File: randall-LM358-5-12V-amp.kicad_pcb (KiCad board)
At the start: 2 copper layers, 137.2 x 91.4 mm, 27 parts, among them J1 Barrel_Jack, M1 Fan_3pin, M2 Fan_3pin, Q1 TIP120, Q2 TIP120, U1 LM2674M-3.3, U2 LM358, U3 Z-Uno

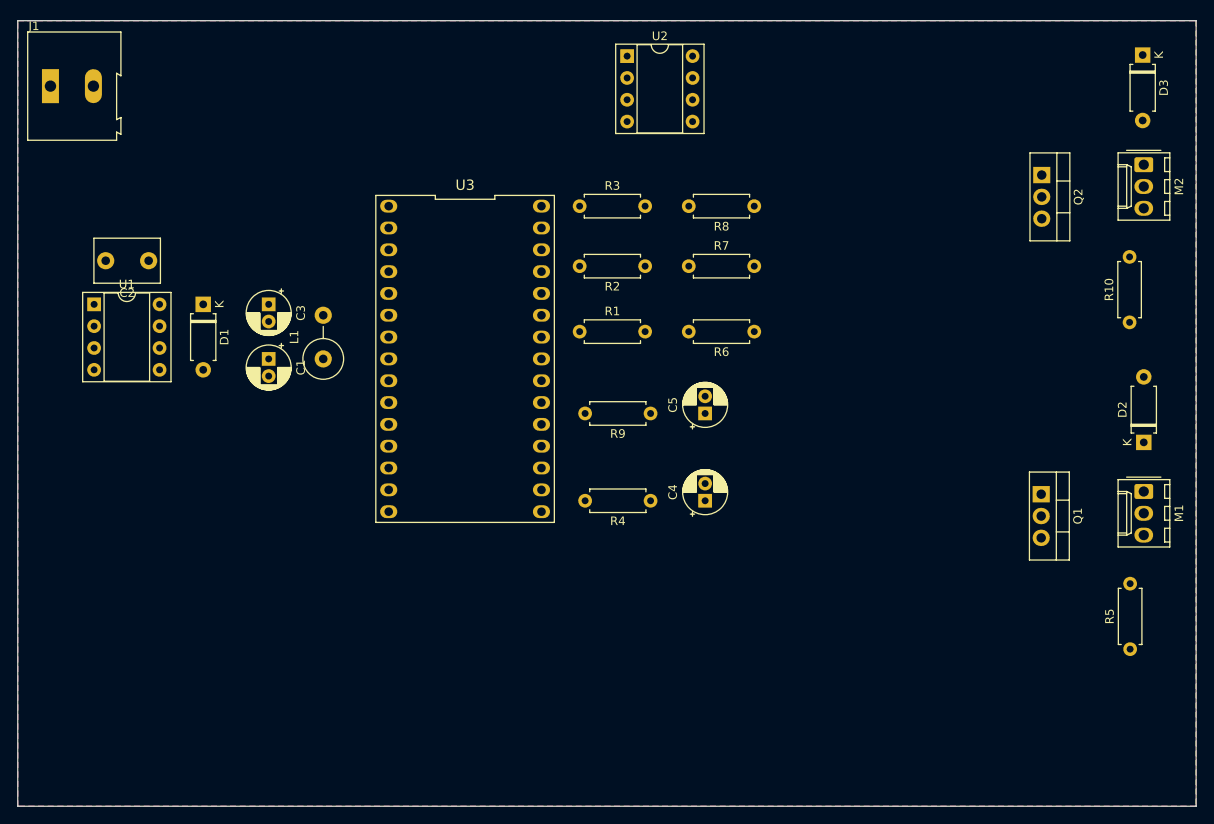
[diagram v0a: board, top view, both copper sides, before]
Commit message: This is it, make no mistake about it
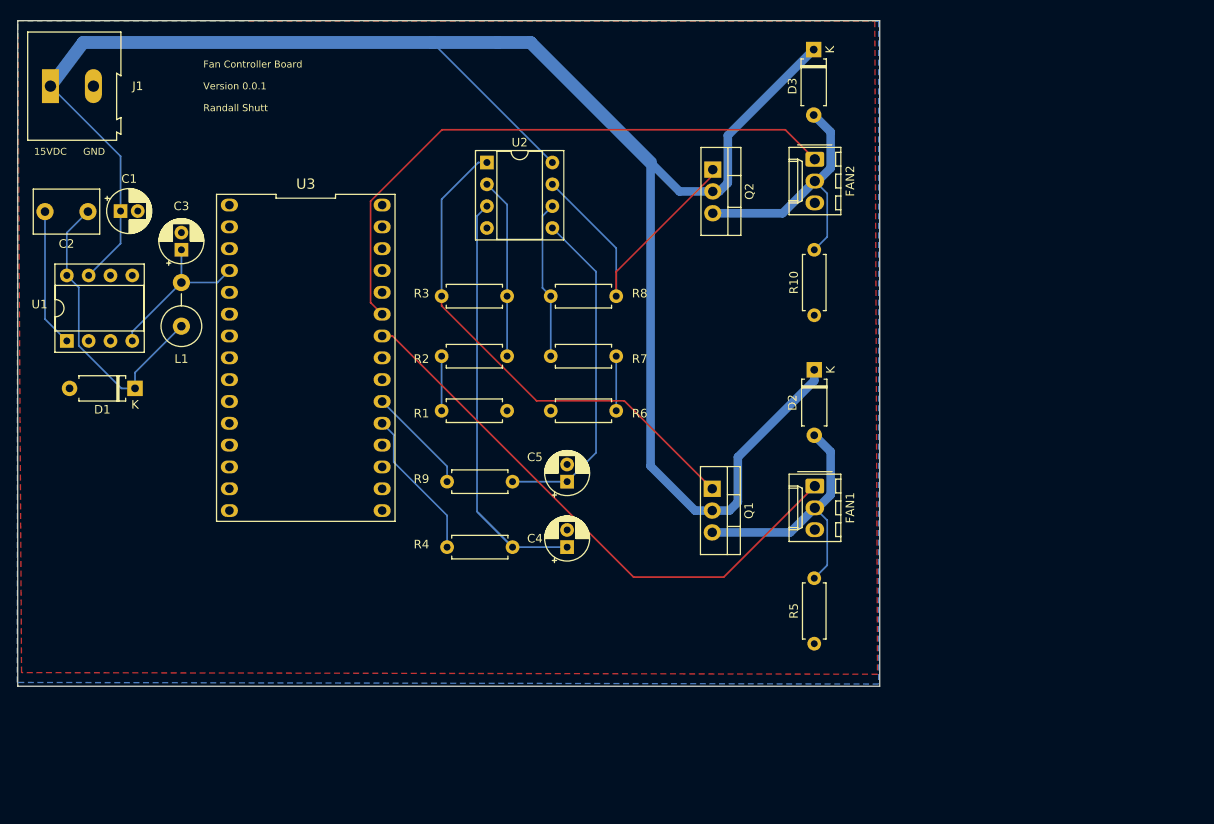
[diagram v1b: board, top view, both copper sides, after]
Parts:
- J1: value Barrel_Jack -> Power
- moved D2 39.3 mm to (175.3, 100.3), turned to 270 degrees
- moved D3 38.3 mm to (175.2, 63.1)
- moved FAN1 38.3 mm to (175.3, 113.9)
- moved FAN2 38.3 mm to (175.3, 75.8)
- moved Q1 38.3 mm to (163.4, 114.2)
- moved Q2 38.3 mm to (163.4, 77.0)
- moved R5 36.8 mm to (175.3, 132.2)
- moved R10 36.7 mm to (175.3, 94.0)
- moved C1 24.4 mm to (94.5, 81.9), turned to 0 degrees
- moved U2 20.5 mm to (137.2, 76.2)
- moved R7 19.2 mm to (144.6, 98.7)
- moved R3 19.2 mm to (131.9, 91.8)
- moved R8 19.2 mm to (152.2, 91.8)
- moved R2 19.2 mm to (139.5, 98.7)
- moved U3 18.5 mm to (116.1, 98.9)
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- renumbered M1 to FAN1, M2 to FAN2
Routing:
- net 15VDC: track 0.00 -> 223.0 mm
- net TACH2: track 0.00 -> 70.3 mm
- net TACH1: track 0.00 -> 66.4 mm
- net Net-(Q1-Pad1): track 0.00 -> 59.8 mm
- net Net-(C4-Pad1): track 0.00 -> 53.9 mm
- net Net-(C5-Pad1): track 0.00 -> 39.4 mm
- net Net-(Q2-Pad1): track 0.00 -> 35.5 mm
- net Net-(C2-Pad1): track 0.00 -> 35.3 mm
- net Net-(D2-Pad2): track 0.00 -> 32.7 mm
- net Net-(D3-Pad2): track 0.00 -> 32.1 mm
- net Net-(R2-Pad1): track 0.00 -> 21.0 mm
- net 3V3DC: track 0.00 -> 19.1 mm
- net Net-(R7-Pad1): track 0.00 -> 18.3 mm
- net PWM1: track 0.00 -> 17.5 mm
- net Net-(C2-Pad2): track 0.00 -> 16.1 mm
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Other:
- board size 137.2 x 91.4 mm -> 100.3 x 77.5 mm
- net class Default: clearance 0.2 -> 0.25; trace_width 0.25 -> 0.127; via_dia 0.8 -> 0.6; via_drill 0.4 -> 0.3
- net class High removed
- rule trace_clearance: 0.2 -> 0.25
- rule trace_min: 0.2 -> 0.127
- rule via_min_size: 0.4 -> 0.6
- board text added: "15VDC"
- board text added: "Fan Controller Board"
- board text added: "GND"
- board text added: "Randall Shutt"
- board text added: "Version 0.0.1"
